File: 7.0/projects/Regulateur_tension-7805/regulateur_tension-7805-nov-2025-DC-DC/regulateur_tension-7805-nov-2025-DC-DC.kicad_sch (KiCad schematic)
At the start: 3 parts, among them J1 Screw_Terminal_01x02, J2 Screw_Terminal_01x02, U1 L7805

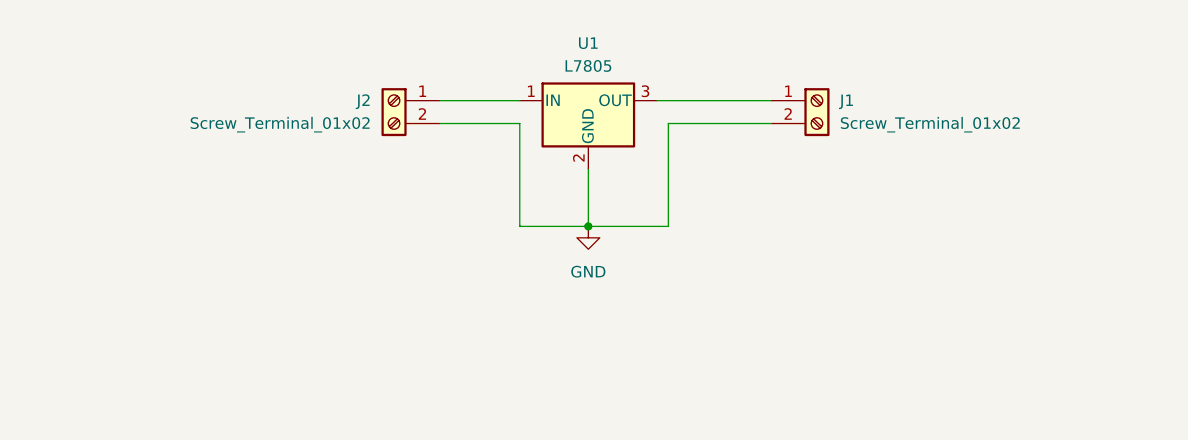
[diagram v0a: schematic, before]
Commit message: adding fuses
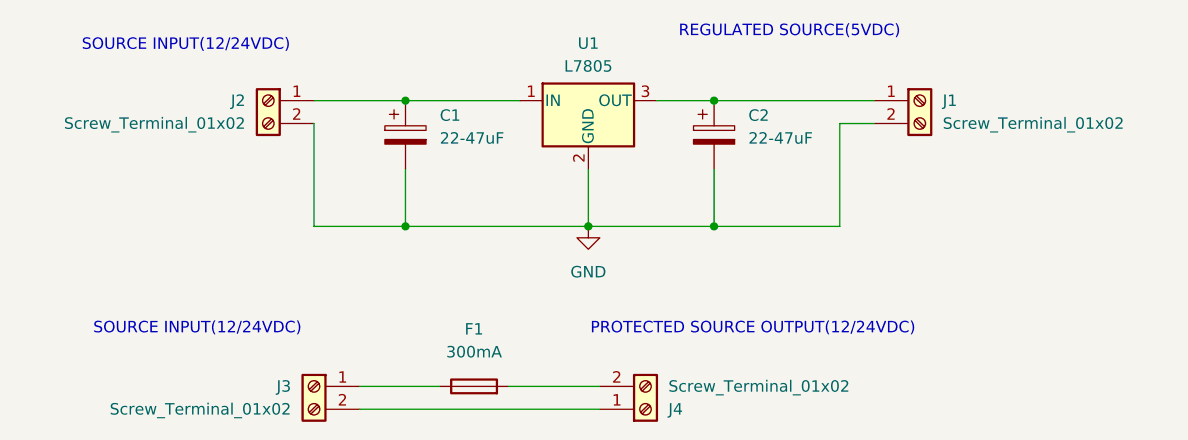
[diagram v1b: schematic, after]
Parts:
- added C1, C2: 22-47uF, symbol Device:C_Polarized
- added F1: 300mA, symbol Device:Fuse
- added J3, J4: Screw_Terminal_01x02, symbol Connector:Screw_Terminal_01x02
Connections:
- net GND: now also C1.2, C2.2
- net at J2.1 (Pin_1), U1.1 (IN): now also C1.1
- net at J1.1 (Pin_1), U1.3 (OUT): now also C2.1
- new net: J3.2 (Pin_2), J4.1 (Pin_1)
- new net: F1.2, J4.2 (Pin_2)
- new net: F1.1, J3.1 (Pin_1)
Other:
- note added: "PROTECTED SOURCE OUTPUT(12/24VDC)"
- note added: "REGULATED SOURCE(5VDC)"
- note added: "SOURCE INPUT(12/24VDC)"
- moved on the sheet: J1, J2
